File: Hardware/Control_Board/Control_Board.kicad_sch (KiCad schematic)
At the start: 2 parts, among them U1 ESP32-S2, U3 DRV8231ADSG

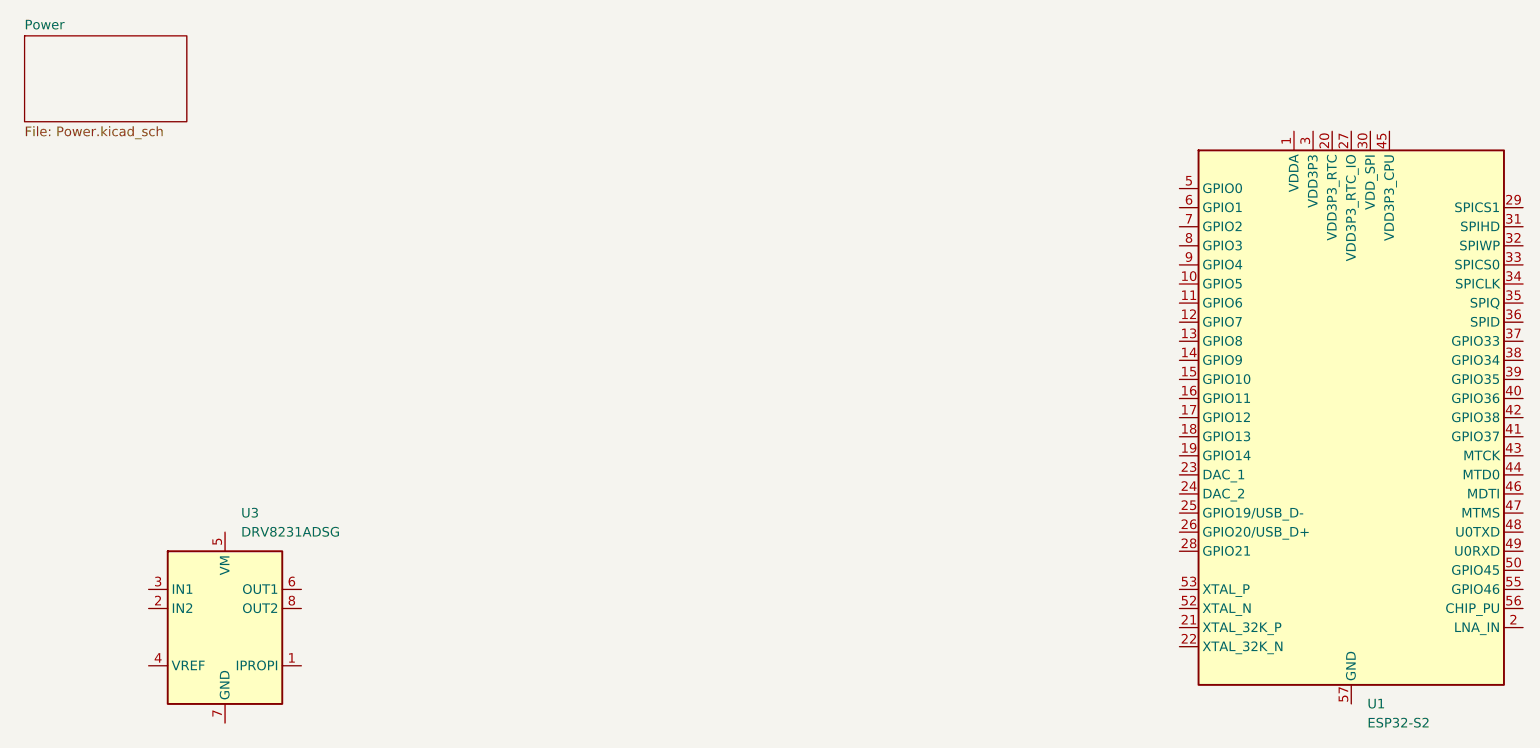
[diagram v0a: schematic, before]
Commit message: fleshed out info/planning, roughed in more schematics, added short readme
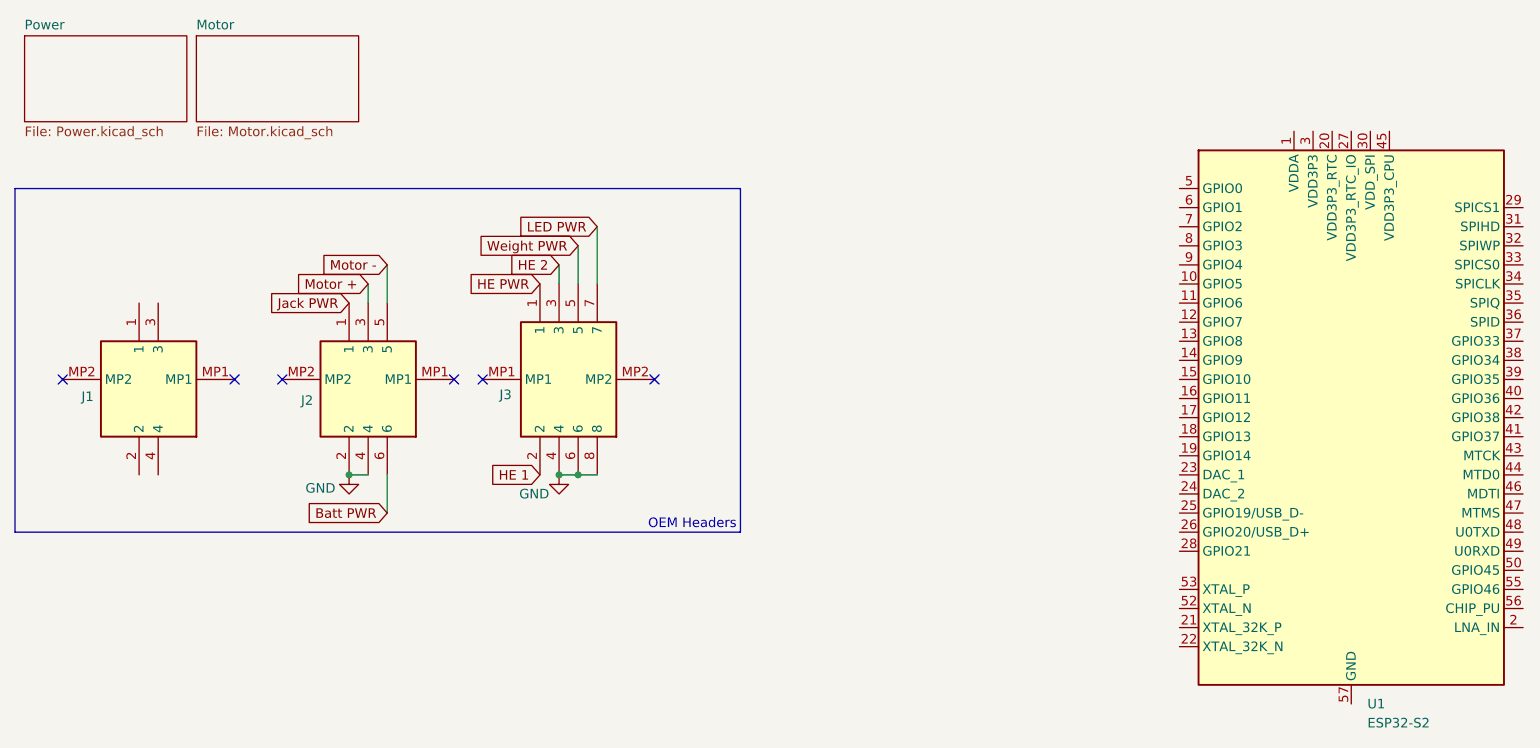
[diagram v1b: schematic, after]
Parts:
- removed U3: DRV8231ADSG, Package_SON:WSON-8-1EP_2x2mm_P0.5mm_EP0.9x1.6mm, symbol Driver_Motor:DRV8231ADSG
- added J1: DF11CZ-4DP-2V_27_, Meow:DF11CZ4DP2V27, symbol Meow:DF11CZ-4DP-2V_27_
- added J2: DF11CZ-4DP-2V_27_, Meow:DF11CZ6DP2V27, symbol Meow:DF11CZ-6DP-2V_27_
- added J3: DF11CZ-8DP-2V_27_, Meow:DF11CZ8DP2V27, symbol Meow:DF11CZ-8DP-2V_27_
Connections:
- new net Batt PWR: J2.6
- new net GND: J2.2, J2.4, J3.4, J3.6, J3.8
- new net HE 1: J3.2
- new net HE 2: J3.3
- new net HE PWR: J3.1
- new net Jack PWR: J2.1
- new net LED PWR: J3.7
- new net Motor +: J2.3
- new net Motor -: J2.5
- new net Weight PWR: J3.5
- no-connect marks 0 -> 6
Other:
- added sheet Motor (Motor.kicad_sch)
- note added: "OEM Headers"
